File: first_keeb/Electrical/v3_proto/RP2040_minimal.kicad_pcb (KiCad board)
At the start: 2 copper layers, 76 x 76 mm, 67 parts, among them P1 USB4105-GF-A, Q1 BSS138, SW1 SW_Push, SW2 SW_Push, U1 NCP1117-3.3_SOT223, U2 LM4040DBZ-3, U3 PRTR5V0U2X, U4 W25Q32JVSS, U5 RP2040, Y1 ABM7-12.000MHZ-D2Y-T

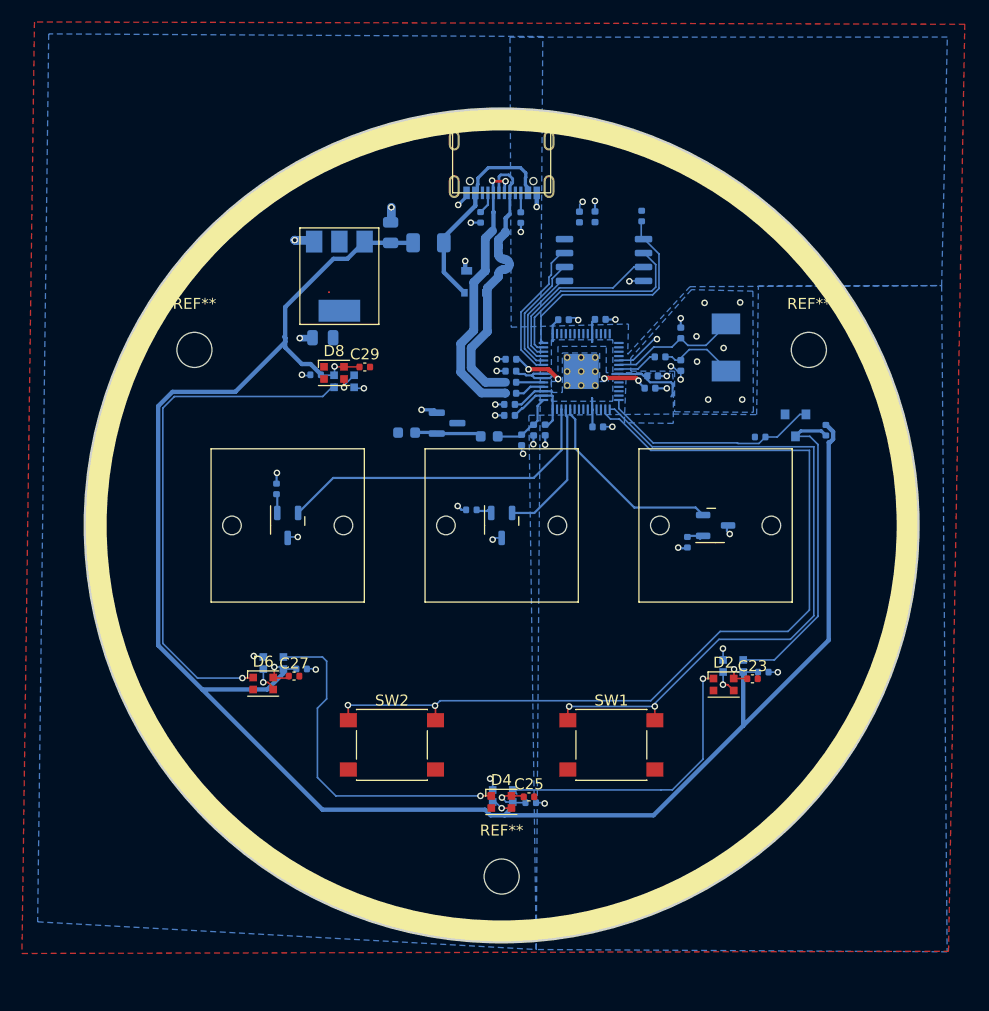
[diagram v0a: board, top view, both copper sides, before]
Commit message: finishes pcb even more
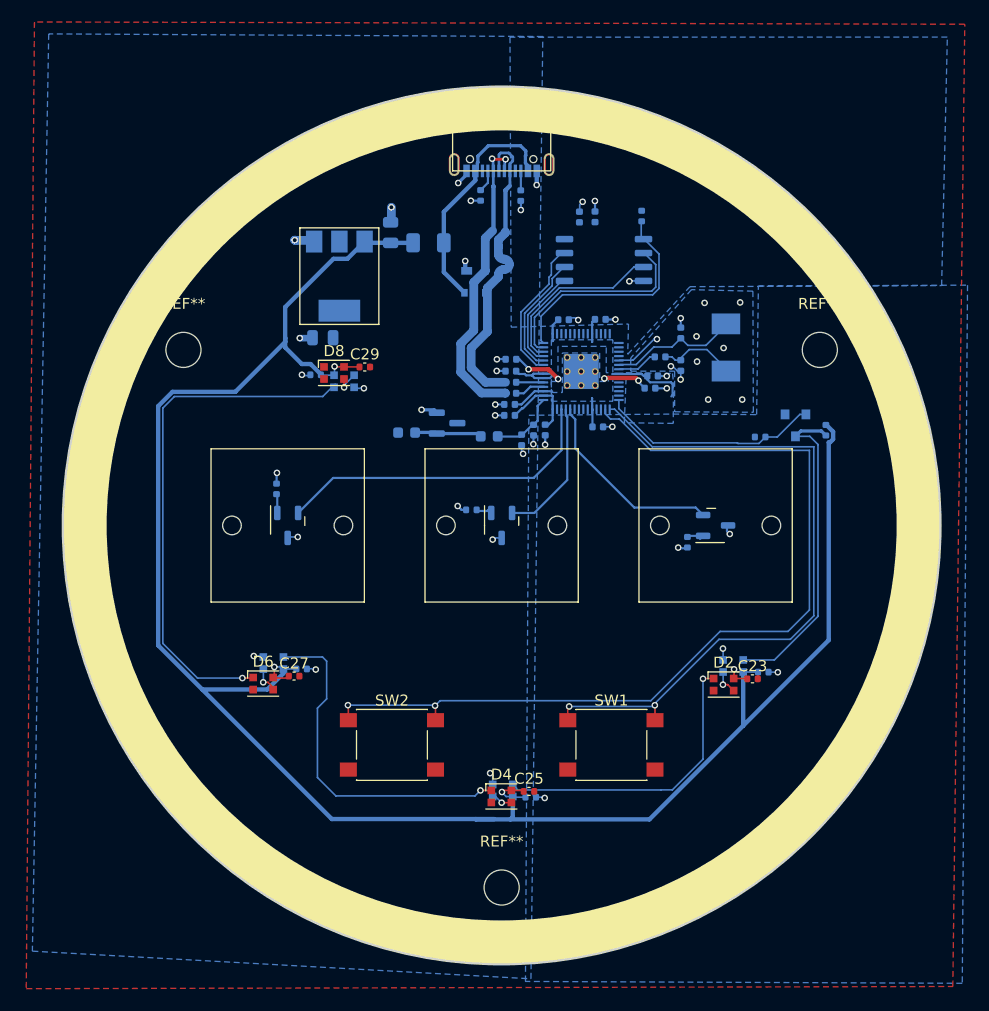
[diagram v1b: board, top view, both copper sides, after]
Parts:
- moved P1 2.00 mm to (100.0, 64.0)
- moved R2 2.00 mm to (98.1, 69.9)
- moved R3 2.00 mm to (101.7, 69.9)
- moved REF** 1.00 mm to (100.0, 133.0)
- moved REF** 1.00 mm to (71.0, 84.0)
- moved REF** 1.00 mm to (129.0, 84.0)
- moved C24 0.50 mm to (102.7, 124.8)
- moved C25 0.50 mm to (102.5, 124.2)
- moved D3 0.50 mm to (100.1, 124.2)
- moved D4 0.50 mm to (100.0, 124.7)
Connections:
- net /GPIO17 renamed GPIO17
- net BUTT0 renamed GPIO18
- net BUTT1 renamed GPIO19
- net GPIO12 renamed /GPIO12
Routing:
- net +5V: track 185.0 -> 187.5 mm
- net /USB_D-: track 25.1 -> 27.5 mm
- net /USB_D+: track 25.9 -> 28.1 mm
- net VBUS: track 19.7 -> 21.4 mm
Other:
- board size 76 x 76 mm -> 80 x 80 mm
